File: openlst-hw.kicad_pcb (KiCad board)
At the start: 4 copper layers, 50 x 43 mm, 65 parts, among them J3 Conn_02x10_Odd_Even, J6 ANT, U2 CC1110, U4 ASFL1-27.000MHZ, U5 MIC803, U6 PE4250, U7 RFFM6406, U8 SF2446E

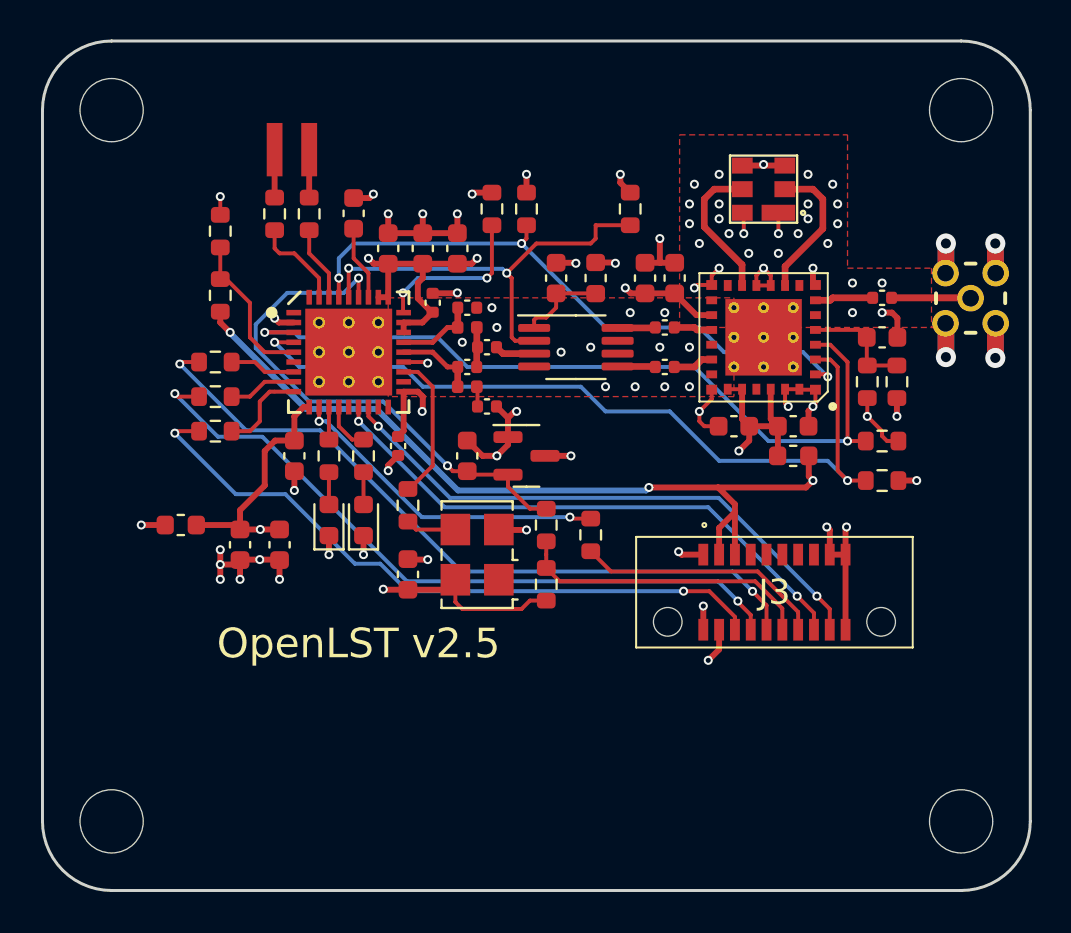
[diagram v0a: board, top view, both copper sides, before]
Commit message: finished edits v2
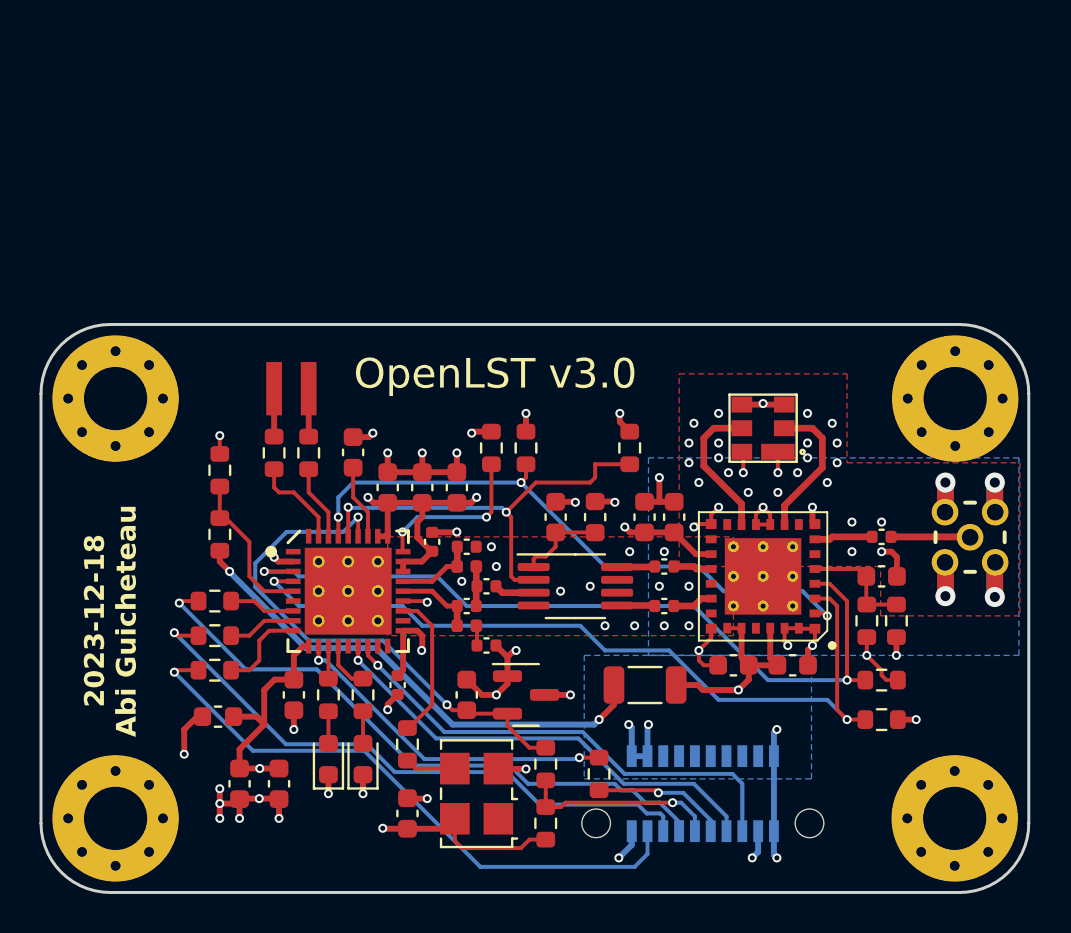
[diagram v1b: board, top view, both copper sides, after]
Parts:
- H1, H2, H3, H4: footprint MountingHole:MountingHole_3.2mm_M3 -> MountingHole:MountingHole_3.2mm_M3_Pad_Via
- J3: moved to B.Cu
- L2: footprint Inductor_SMD:L_0603_1608Metric -> Inductor_SMD:L_1206_3216Metric
- moved H3 45.2 mm to (141.0, 90.5)
- moved H4 45.1 mm to (183.5, 90.5)
- moved L2 13.8 mm to (167.8, 105.0), turned to 0 degrees
- moved R8 12.1 mm to (165.5, 109.5)
- moved C1 12.1 mm to (150.0, 105.5)
- moved C10 12.1 mm to (158.3, 95.0)
- moved C11 12.1 mm to (169.3, 96.5)
- moved C19 12.1 mm to (153.0, 93.2)
- moved C2 12.1 mm to (155.3, 105.0)
- moved C21 12.1 mm to (159.8, 103.0)
- moved C22 12.1 mm to (158.8, 105.5)
- moved C23 12.1 mm to (158.8, 98.0)
- moved C24 12.1 mm to (158.8, 101.0)
- moved C25 12.1 mm to (159.8, 100.0)
- moved C26 12.1 mm to (163.3, 96.5)
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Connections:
- J3 pad 10: /UART_CTS_1 -> /UART_RX_1
- J3 pad 14: /UART_RX_1 -> /UART_CTS_1
- J3 pad 16: /PROG_DD -> /UART_RTS_1
- J3 pad 18: /PROG_DC -> /UART_TX_1
- J3 pad 6: /UART_TX_1 -> /PROG_DC
- J3 pad 8: /UART_RTS_1 -> /PROG_DD
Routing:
- net VAA: track 41.9 -> 25.4 mm, vias 3 -> 2
- net /UART_RX_1: track 12.7 -> 6.83 mm, vias 0 -> 1
- net /UART_CTS_1: track 37.0 -> 31.4 mm, vias 2 -> 1
- net /PROG_DD: track 28.6 -> 23.4 mm, vias 2 -> 1
- net /UART_RTS_1: track 35.9 -> 30.6 mm, vias 2 -> 1
- net /~{LST_RESET}: track 15.2 -> 10.0 mm, vias 0 -> 1
- net /PROG_DC: track 28.9 -> 24.5 mm, vias 2 -> 1
- net /UART_TX_1: track 34.3 -> 30.7 mm, vias 2 -> 1
- net GND: track 78.3 -> 80.7 mm, vias 78 -> 79
- net /VAA_FILT: track 14.1 -> 15.9 mm
- net +3V3: track 18.5 -> 19.5 mm
- added copper zone on B.Cu, net GND
- added copper zone on B.Cu, net VAA
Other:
- board size 50 x 43 mm -> 50 x 28.7 mm
- board text added: "2023-12-18 Abi Guicheteau"
- board text added: "OpenLST v3.0"
- board text removed: "OpenLST v2.5"
